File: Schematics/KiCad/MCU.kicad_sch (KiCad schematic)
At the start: 24 parts, among them J12 B5B-EH-A(LF)(SN), SW1 2-1977223-2, U10 STM32F446RET6, U16 LD1117S33CTR, Y1 ABLS-8.000MHZ-B2-T

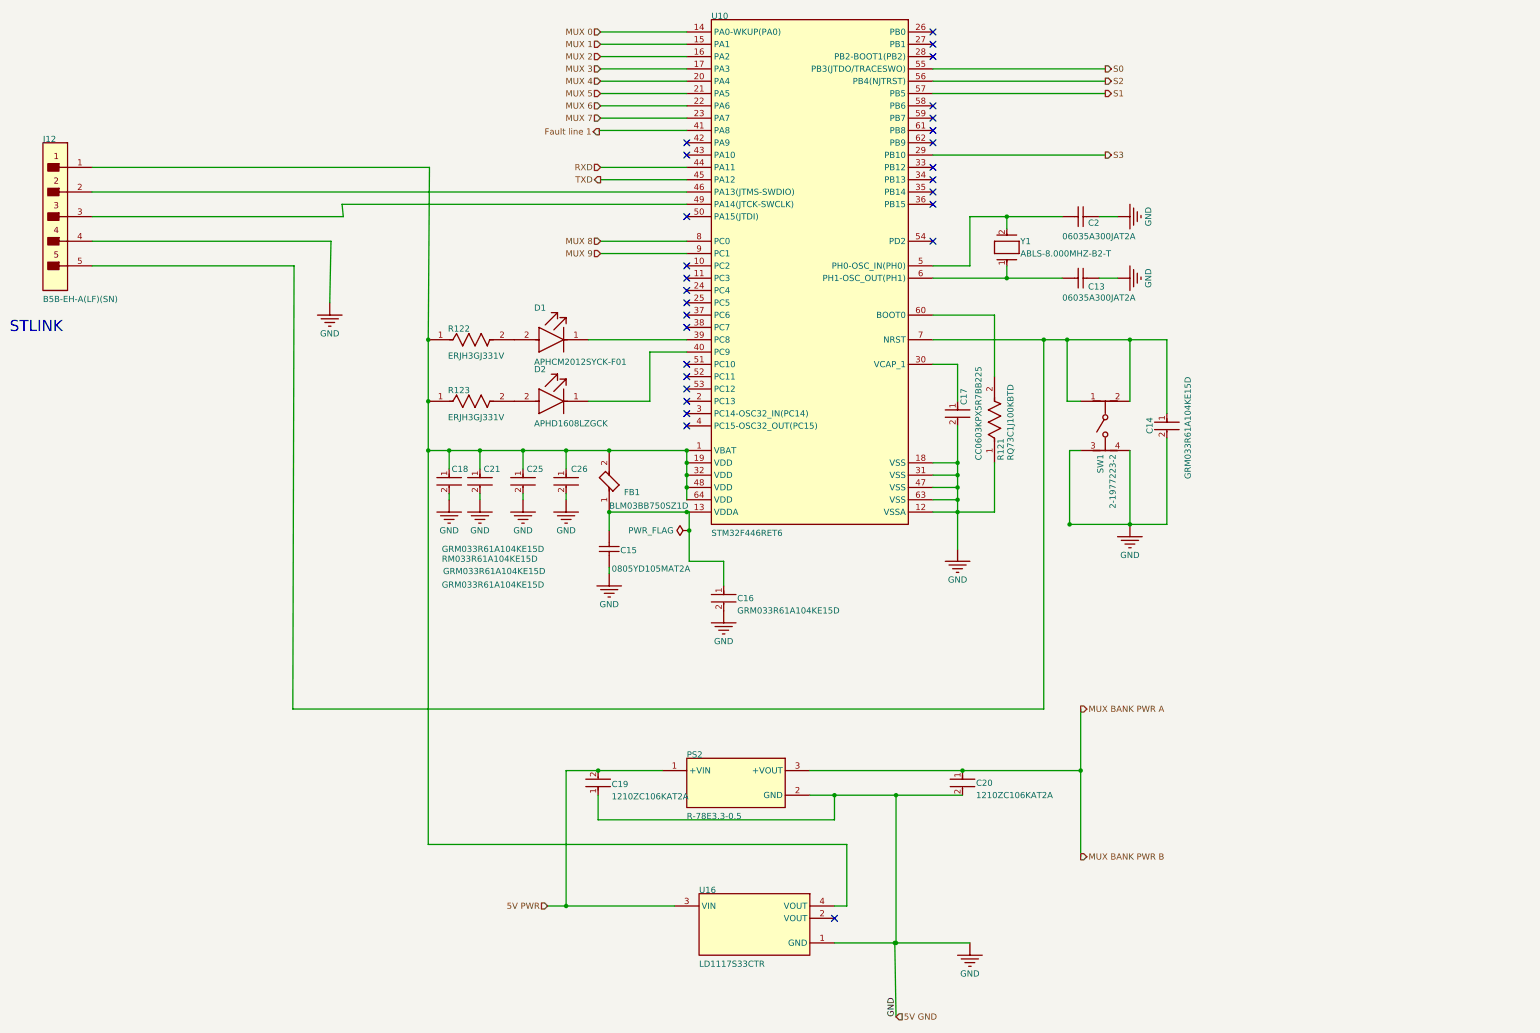
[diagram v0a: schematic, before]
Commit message: Fix all errors and warnings
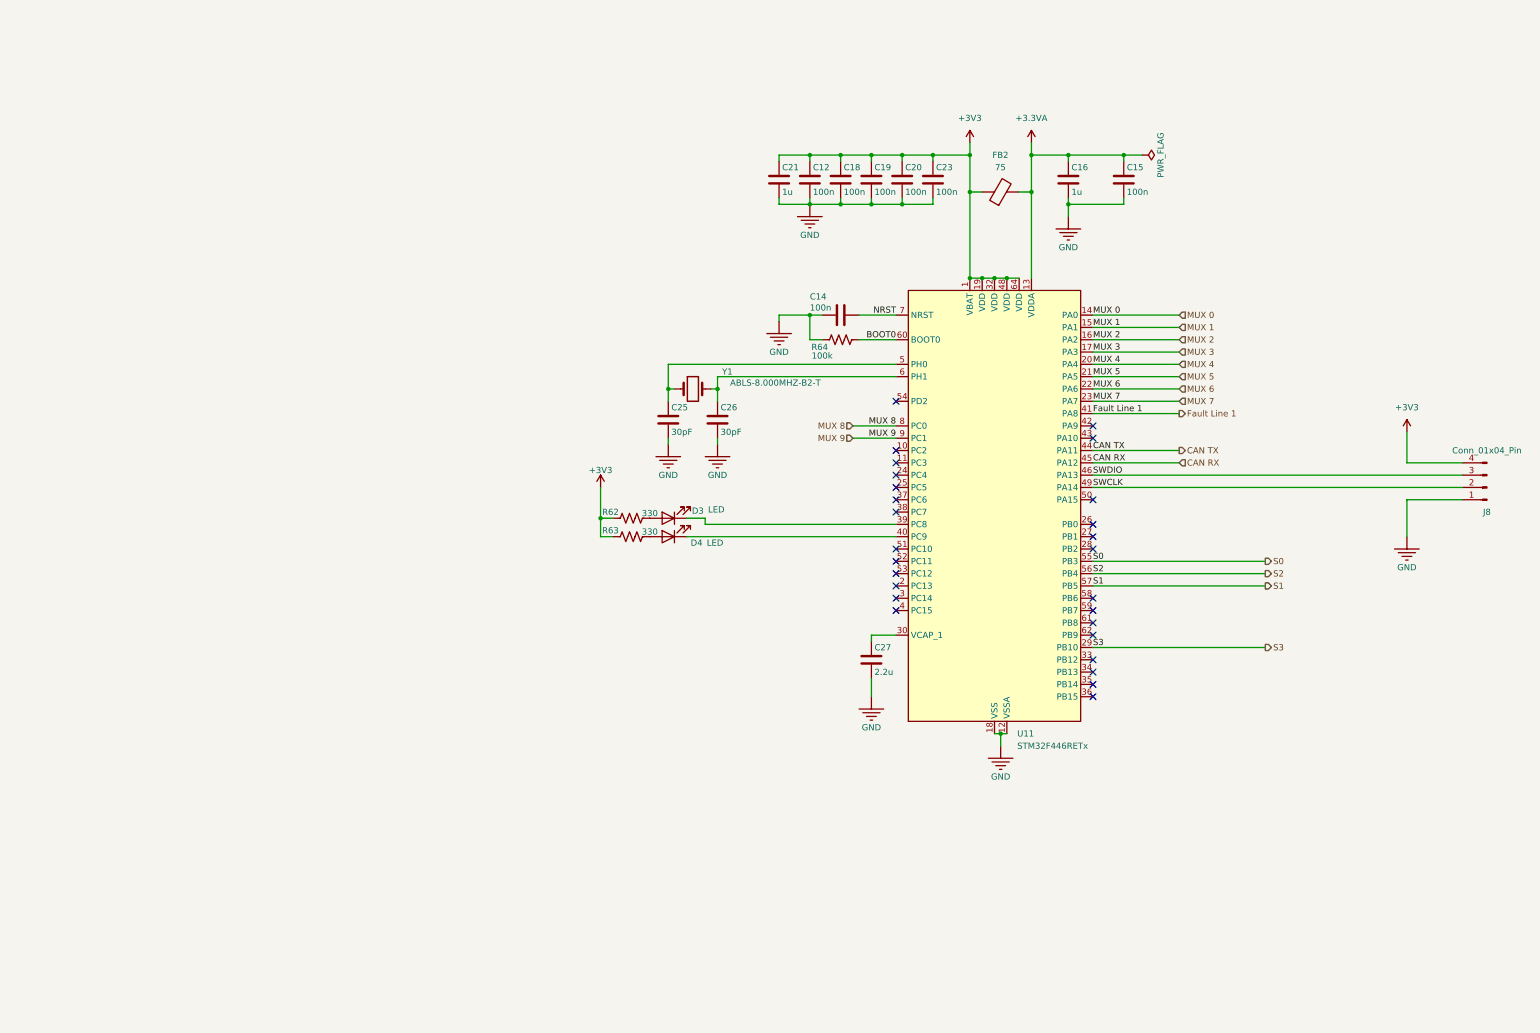
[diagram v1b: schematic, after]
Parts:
- removed C13, C2: 06035A300JAT2A, CAPC1608X90X35LL15T15, symbol Altium Content Vault:MCU_1_CAP_Altium Content Vault_0
- removed C14: GRM033R61A104KE15D, FP-GRM033-0_03-IPC_C, symbol Altium Content Vault:MCU_1_b4654b650e69147ec39a6b967a45e02_Altium Content Vault
- removed C15: 0805YD105MAT2A, CAPC2013X140X50NL20T25, symbol Altium Content Vault:MCU_1_CAP_Altium Content Vault_0
- removed C16, C18, C25, C26: GRM033R61A104KE15D, FP-GRM033-0_03-IPC_C, symbol Altium Content Vault:MCU_0_b4654b650e69147ec39a6b967a45e02_Altium Content Vault
- removed C17: CC0603KPX5R7BB225, FP-CC0603-DA-MFG, symbol Altium Content Vault:MCU_0_11868f565c42a9108669ba33697ecf6_Altium Content Vault
- removed C19: 1210ZC106KAT2A, FP-1210-L_3_3_0_4-W_2_5_0-IPC_A, symbol Altium Content Vault:MCU_2_b4654b650e69147ec39a6b967a45e02_Altium Content Vault
- removed C20: 1210ZC106KAT2A, FP-1210-L_3_3_0_4-W_2_5_0-IPC_A, symbol Altium Content Vault:MCU_0_b4654b650e69147ec39a6b967a45e02_Altium Content Vault
- removed C21: RM033R61A104KE15D, FP-GRM033-0_03-IPC_C, symbol Altium Content Vault:MCU_0_b4654b650e69147ec39a6b967a45e02_Altium Content Vault
- removed D1: APHCM2012SYCK-F01, FP-APHCM2012SYCK-F01-MFG, symbol Altium Content Vault:MCU_0_8706943c75ba83719d021d2fdc84c58_Altium Content Vault
- removed D2: APHD1608LZGCK, FP-APHD1608LZGCK-MFG, symbol Altium Content Vault:MCU_0_8706943c75ba83719d021d2fdc84c58_Altium Content Vault
- removed FB1: BLM03BB750SZ1D, FP-BLM03-0_03-d0_3-IPC_C, symbol Altium Content Vault:MCU_0_5f30dd21d616792df468990f7003faa_Altium Content Vault
- removed J12: B5B-EH-A(LF)(SN), FP-B5B-EH-A_LF_SN-MFG, symbol Altium Content Vault:MCU_0_bf93c07fd2649a848d0ec8585582aab_Altium Content Vault
- removed PS2: R-78E3.3-0.5, CONV_R-78E3.3-0.5, symbol R-78E3.3-0.5:MCU_0_R-78E3.3-0.5_R-78E3.3-0.5.IntLib
- removed R121: RQ73C1J100KBTD, FP-RQ731J-IPC_C, symbol Altium Content Vault:MCU_1_1029c3af85768c4190bb7ad29bc67b5_Altium Content Vault
- removed R122, R123: ERJH3GJ331V, FP-ERJH3G-MFG, symbol Altium Content Vault:MCU_0_1029c3af85768c4190bb7ad29bc67b5_Altium Content Vault
- removed SW1: 2-1977223-2, FP-2-1977223-2-MFG, symbol Altium Content Vault:MCU_0_b8895f3f4cefb76e1819d2863dba89b_Altium Content Vault
- removed U10: STM32F446RET6, STM-LQFP64_L, symbol Altium Content Vault:MCU_0_MC-ARM-STM32F446-LQFP64_Altium Content Vault
- removed U16: LD1117S33CTR, FP-SOT-223-0046067_14-MFG, symbol Altium Content Vault:MCU_0_7818869c5c16ceab15634627166a29d_Altium Content Vault
- removed Y1: ABLS-8.000MHZ-B2-T, FP-ABLS-MFG, symbol Altium Content Vault:MCU_1_c23a69dc6c9e2f18f2079038eb95dd1_Altium Content Vault
- added C12, C14, C15, C18, C19, C20, C23: 100n, Capacitor_SMD:C_0603_1608Metric, symbol Device:C
- added C16, C21: 1u, Capacitor_SMD:C_0603_1608Metric, symbol Device:C
- added C25, C26: 30pF, Capacitor_SMD:C_0603_1608Metric, symbol Device:C
- added C27: 2.2u, Capacitor_SMD:C_0603_1608Metric, symbol Device:C
- added D3, D4: LED, symbol Device:LED
- added FB2: 75, Resistor_SMD:R_0603_1608Metric, symbol Device:FerriteBead
- added J8: Conn_01x04_Pin, symbol Connector:Conn_01x04_Pin
- added R62, R63: 330, Resistor_SMD:R_0603_1608Metric, symbol Device:R_US
- added R64: 100k, Resistor_SMD:R_0603_1608Metric, symbol Device:R_US
- added U11: STM32F446RETx, Package_QFP:LQFP-64_10x10mm_P0.5mm, symbol MCU_ST_STM32F4:STM32F446RETx
- added Y1: ABLS-8.000MHZ-B2-T, symbol Device:Crystal
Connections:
- net GND: now also C12.2, C14.2, C15.2, C16.2, C18.2, C19.2, C20.2, C21.2, C23.2, C25.2, C26.2, C27.2, J8.1 (Pin_1), R64.2, U11.12 (VSSA), U11.18 (VSS), U11.31 (VSS), U11.47 (VSS), U11.63 (VSS)
- net MUX 0: now also U11.14 (PA0)
- net MUX 1: now also U11.15 (PA1)
- net MUX 2: now also U11.16 (PA2)
- net MUX 3: now also U11.17 (PA3)
- net MUX 4: now also U11.20 (PA4)
- net MUX 5: now also U11.21 (PA5)
- net MUX 6: now also U11.22 (PA6)
- net MUX 7: now also U11.23 (PA7)
- net MUX 8: now also U11.8 (PC0)
- net MUX 9: now also U11.9 (PC1)
- net S0: now also U11.55 (PB3)
- net S1: now also U11.57 (PB5)
- net S2: now also U11.56 (PB4)
- net S3: now also U11.29 (PB10)
- new net: C27.1, U11.30 (VCAP_1)
- new net: D3.2 (A), R62.2
- new net: D3.1 (K), U11.39 (PC8)
- new net: D4.1 (K), U11.40 (PC9)
- new net: D4.2 (A), R63.2
- new net: C25.1, U11.5 (PH0), Y1.1
- new net: C26.1, U11.6 (PH1), Y1.2
- new net +3.3VA: C15.1, C16.1, FB2.2, U11.13 (VDDA)
- new net +3V3: C12.1, C18.1, C19.1, C20.1, C21.1, C23.1, FB2.1, J8.4 (Pin_4), R62.1, R63.1, U11.1 (VBAT), U11.19 (VDD), U11.32 (VDD), U11.48 (VDD), U11.64 (VDD)
- new net BOOT0: R64.1, U11.60 (BOOT0)
- new net CAN RX: U11.45 (PA12)
- new net CAN TX: U11.44 (PA11)
- new net Fault Line 1: U11.41 (PA8)
- new net NRST: C14.1, U11.7 (NRST)
- new net SWCLK: J8.2 (Pin_2), U11.49 (PA14)
- new net SWDIO: J8.3 (Pin_3), U11.46 (PA13)
- no-connect marks 28 -> 27
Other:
- note removed: "STLINK"
